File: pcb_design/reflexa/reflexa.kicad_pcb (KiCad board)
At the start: 2 copper layers, 93 x 73 mm, 10 parts, among them J1 Conn_02x13_Odd_Even, J2 USB_C_Receptacle, J3 USB_C_Receptacle, J4 USB_C_Receptacle, J5 USB_C_Receptacle

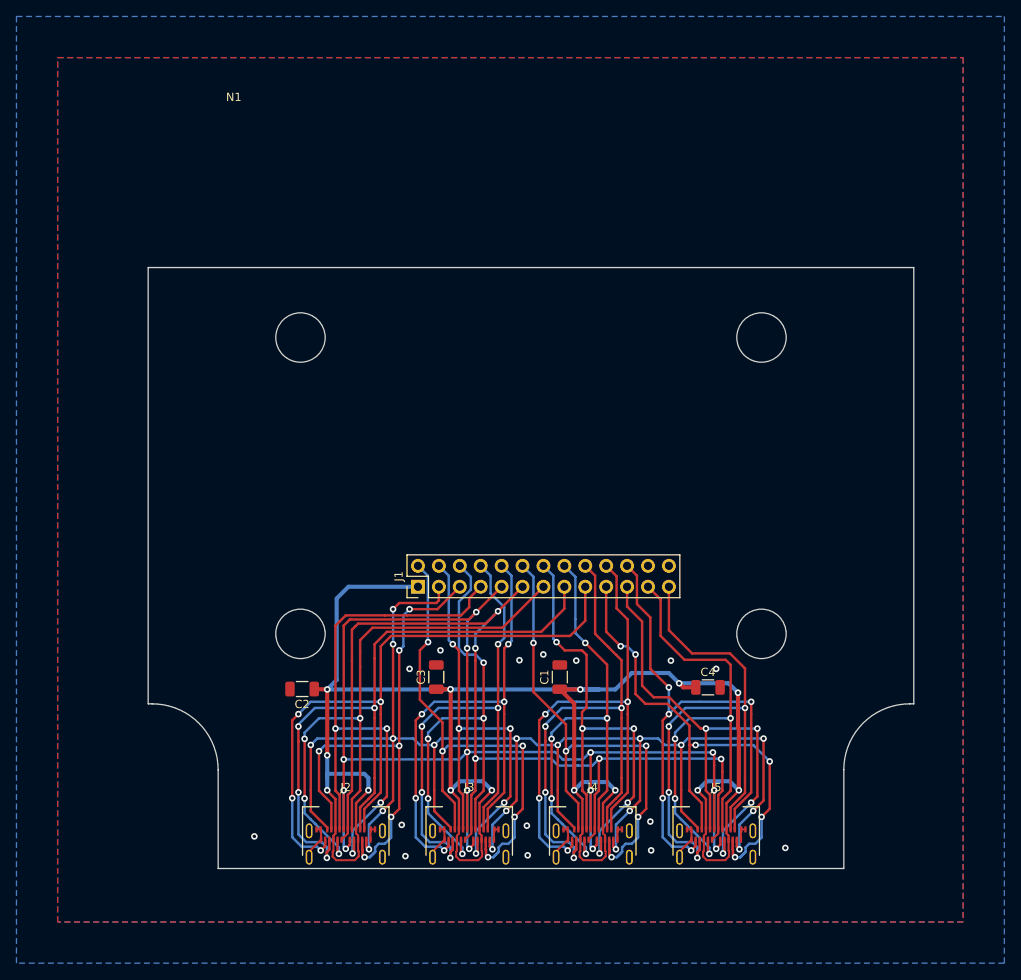
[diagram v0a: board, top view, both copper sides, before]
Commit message: Partial redesign.
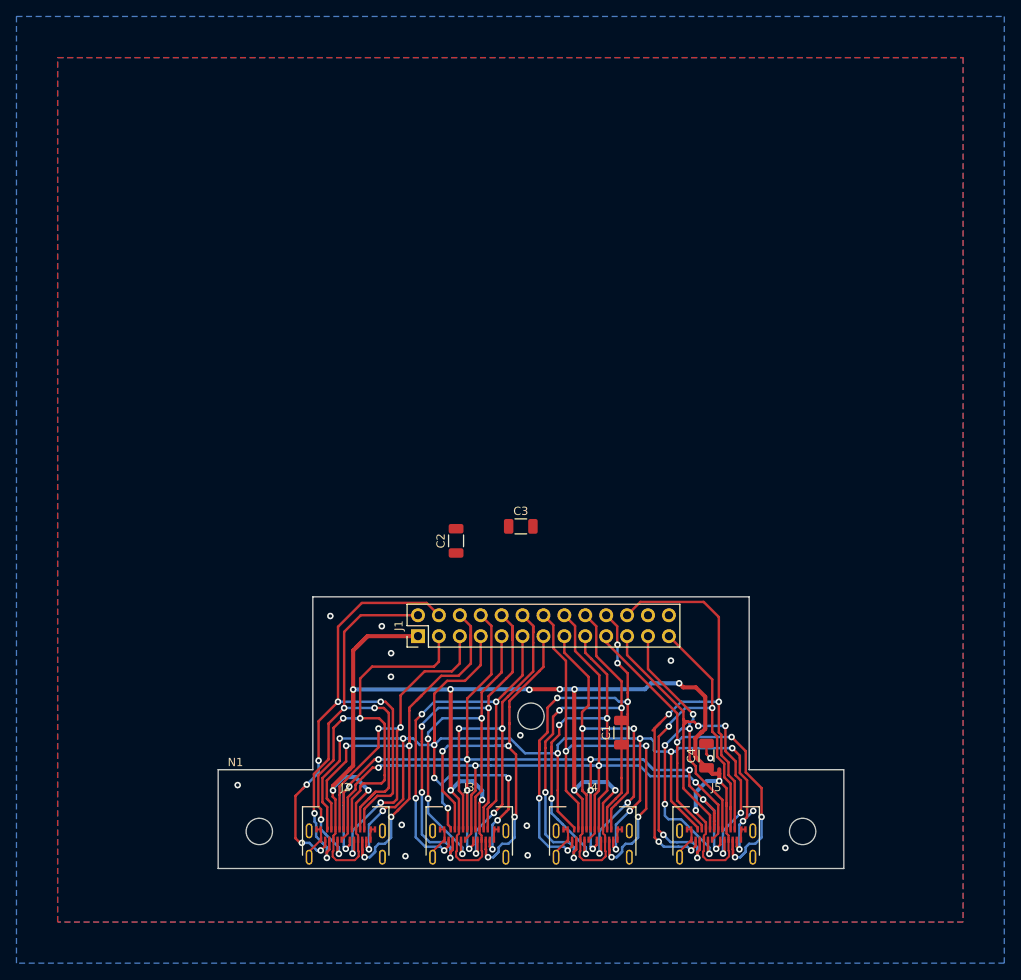
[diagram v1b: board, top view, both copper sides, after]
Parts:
- N1: footprint custom_footprints:Enclosure-Gloxinia2 -> custom_footprints:Enclosure-Gloxinia_front
- moved N1 28.0 mm to (147.5, 100.0)
- moved C2 26.0 mm to (138.4, 78.7), turned to 90 degrees
- moved C3 21.0 mm to (146.3, 76.9), turned to 0 degrees
- moved C1 10.1 mm to (158.5, 102.0)
- moved C4 8.30 mm to (168.8, 104.8), turned to 90 degrees
- moved J1 6.00 mm to (133.8, 90.3)
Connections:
- J1 pad 10: /A11-2 -> /A10-2
- J1 pad 11: /A7 -> /A11-2
- J1 pad 12: /A3-3 -> /A5-2
- J1 pad 13: /A8-1 -> /A3-2
- J1 pad 14: /A5-3 -> /A3-3
- J1 pad 15: /A10-1 -> /A5-3
- J1 pad 16: /A8-3 -> /A7
- J1 pad 17: /A11-1 -> /A8-3
- J1 pad 2: /A3-2 -> /A10-1
- J1 pad 3: /A2 -> /A8-1
- J1 pad 4: /A5-2 -> /A11-1
- J1 pad 5: /A3-1 -> /A5-1
- J1 pad 6: /A8-2 -> /A3-1
- J1 pad 7: /A5-1 -> /A2
- J1 pad 8: /A10-2 -> /A6
- J1 pad 9: /A6 -> /A8-2
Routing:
- net /A6: track 171.5 -> 131.5 mm, vias 14 -> 12
- net /A7: track 129.7 -> 99.2 mm, vias 5 -> 4
- net /PS: track 241.6 -> 215.4 mm
- net /A10-1: track 84.2 -> 67.4 mm
- net /A5-1: track 70.1 -> 53.3 mm
- net /A8-1: track 74.1 -> 59.6 mm
- net /A11-1: track 84.9 -> 71.9 mm, vias 4 -> 6
- net /A8-4: track 62.7 -> 50.0 mm, vias 4 -> 5
- net /A10-4: track 70.2 -> 57.7 mm
- net /A8-2: track 61.3 -> 50.5 mm, vias 5 -> 4
- net /A5-3: track 60.8 -> 50.2 mm, vias 5 -> 4
- net /A3-2: track 66.2 -> 56.6 mm, vias 5 -> 4
- net /A11-2: track 65.2 -> 56.1 mm, vias 5 -> 4
- net /A8-3: track 60.3 -> 51.3 mm, vias 5 -> 4
- net /A3-4: track 66.5 -> 58.8 mm, vias 6 -> 4
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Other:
- board size 93 x 73 mm -> 76 x 33 mm
